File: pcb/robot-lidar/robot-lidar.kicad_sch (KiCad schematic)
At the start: 38 parts, among them J10 Conn_01x18, J11 USB_A, J12 Conn_02x20_Odd_Even, J2 YLIDAR X4, J3 Jack-DC, J5 Conn_01x02, J5 Conn_02x03_Odd_Even, J6 Conn_01x02, J7 Conn_01x02, J7 Conn_ARM_SWD_TagConnect_TC2030, J8 Conn_01x02, J9 Conn_01x18, U1 STM32F103C8Tx, U2 LM317-3.3_SOT-223, U2 MPU-6050, U4 MX1508, U5 MX1508, Y1 Crystal

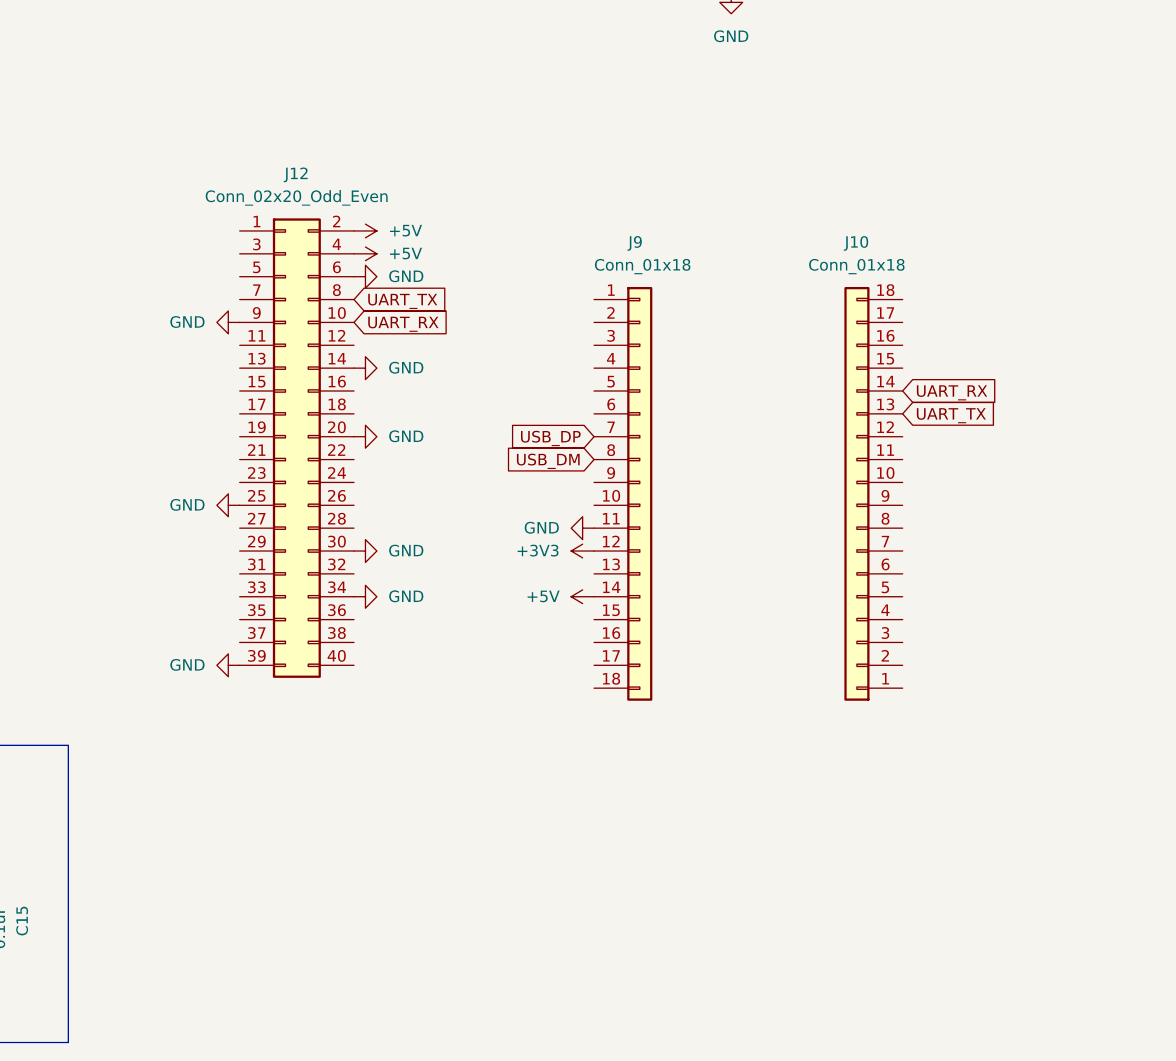
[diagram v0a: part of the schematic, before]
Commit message: saving shematic
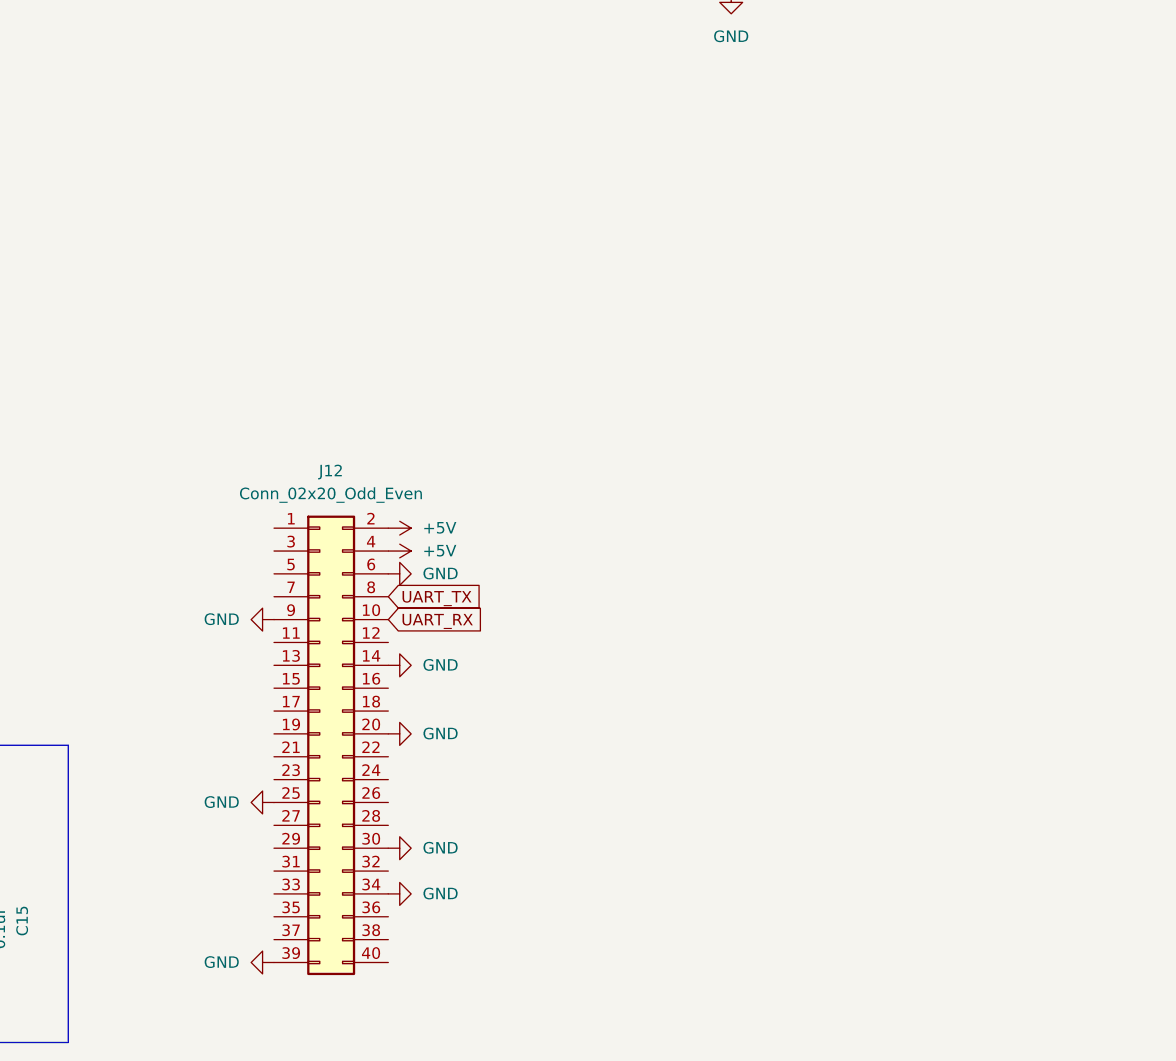
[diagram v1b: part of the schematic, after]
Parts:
- removed J10, J9: Conn_01x18, Connector_PinHeader_2.54mm:PinHeader_1x18_P2.54mm_Vertical, symbol Connector_Generic:Conn_01x18
- J12: footprint (none) -> Connector_PinHeader_2.54mm:PinHeader_2x20_P2.54mm_Vertical
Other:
- moved on the sheet: J12

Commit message: finish V2
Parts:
- removed J11: USB_A, Connector_USB:USB_A_Molex_48037-2200_Horizontal, symbol Connector:USB_A
- removed R13, R14: 10K, Resistor_SMD:R_0603_1608Metric, symbol Device:R
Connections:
- net I2C_SCL is gone; now on net SCL: R1.2, U2.23 (SCL)
- net I2C_SDA is gone; now on net SDA: R2.2, U2.24 (SDA)
- net INT is gone; now on net MOTOR_2_B: U1.18 (PB0)
- net UART4_RX is gone; now on net UART_RX: J2.2 (Pin_2)
- net UART4_TX is gone; now on net UART_TX: J2.3 (Pin_3)
- net DEV_EN: now also J12.29 (Pin_29)
- net MOTOR_1_A: now also U1.16 (PA6); no longer U1.12 (PA2)
- net MOTOR_1_B: now also U1.17 (PA7); no longer U1.13 (PA3)
- net MOTOR_2_A: now also U1.19 (PB1); no longer U1.10 (PA0)
- net MOTOR_2_B: no longer U1.11 (PA1)
- net MOTOR_3_A: now also U1.42 (PB6); no longer U1.16 (PA6)
- net MOTOR_3_B: now also U1.43 (PB7); no longer U1.17 (PA7)
- net MOTOR_4_A: now also U1.45 (PB8); no longer U1.29 (PA8)
- net MOTOR_4_B: now also U1.46 (PB9); no longer U1.30 (PA9)
- net M_EN: now also J12.31 (Pin_31)
- net M_SCTR: now also J12.32 (Pin_32)
- net SCL: now also J12.5 (Pin_5)
- net SDA: now also J12.3 (Pin_3)
